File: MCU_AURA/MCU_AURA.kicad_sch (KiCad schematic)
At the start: 0 parts

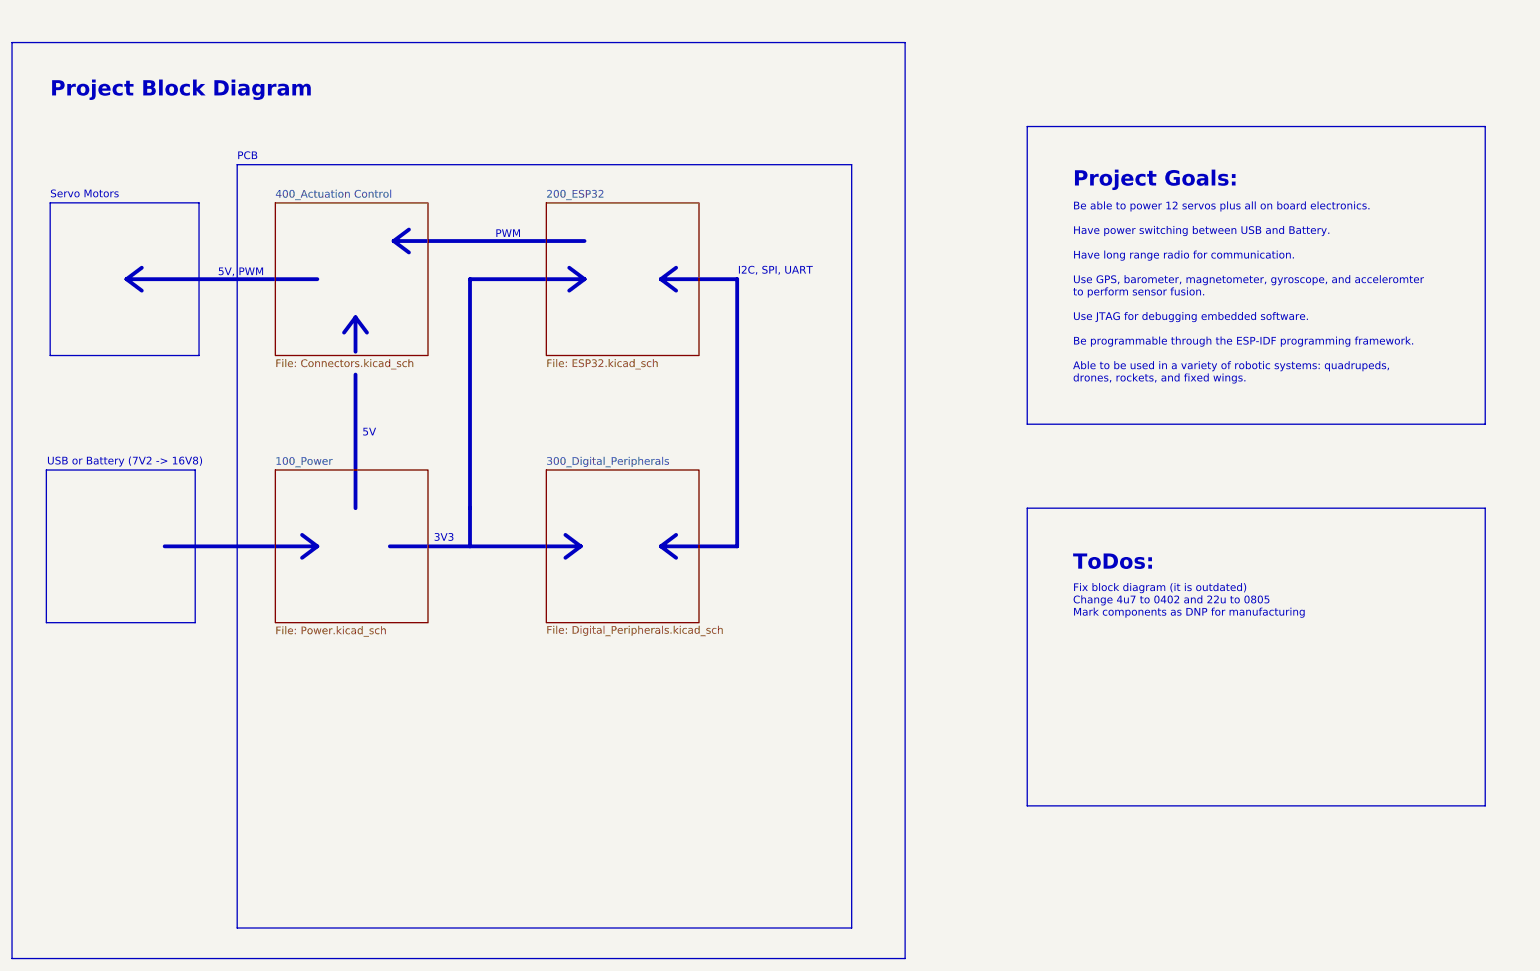
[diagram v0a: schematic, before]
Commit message: First fully routed version
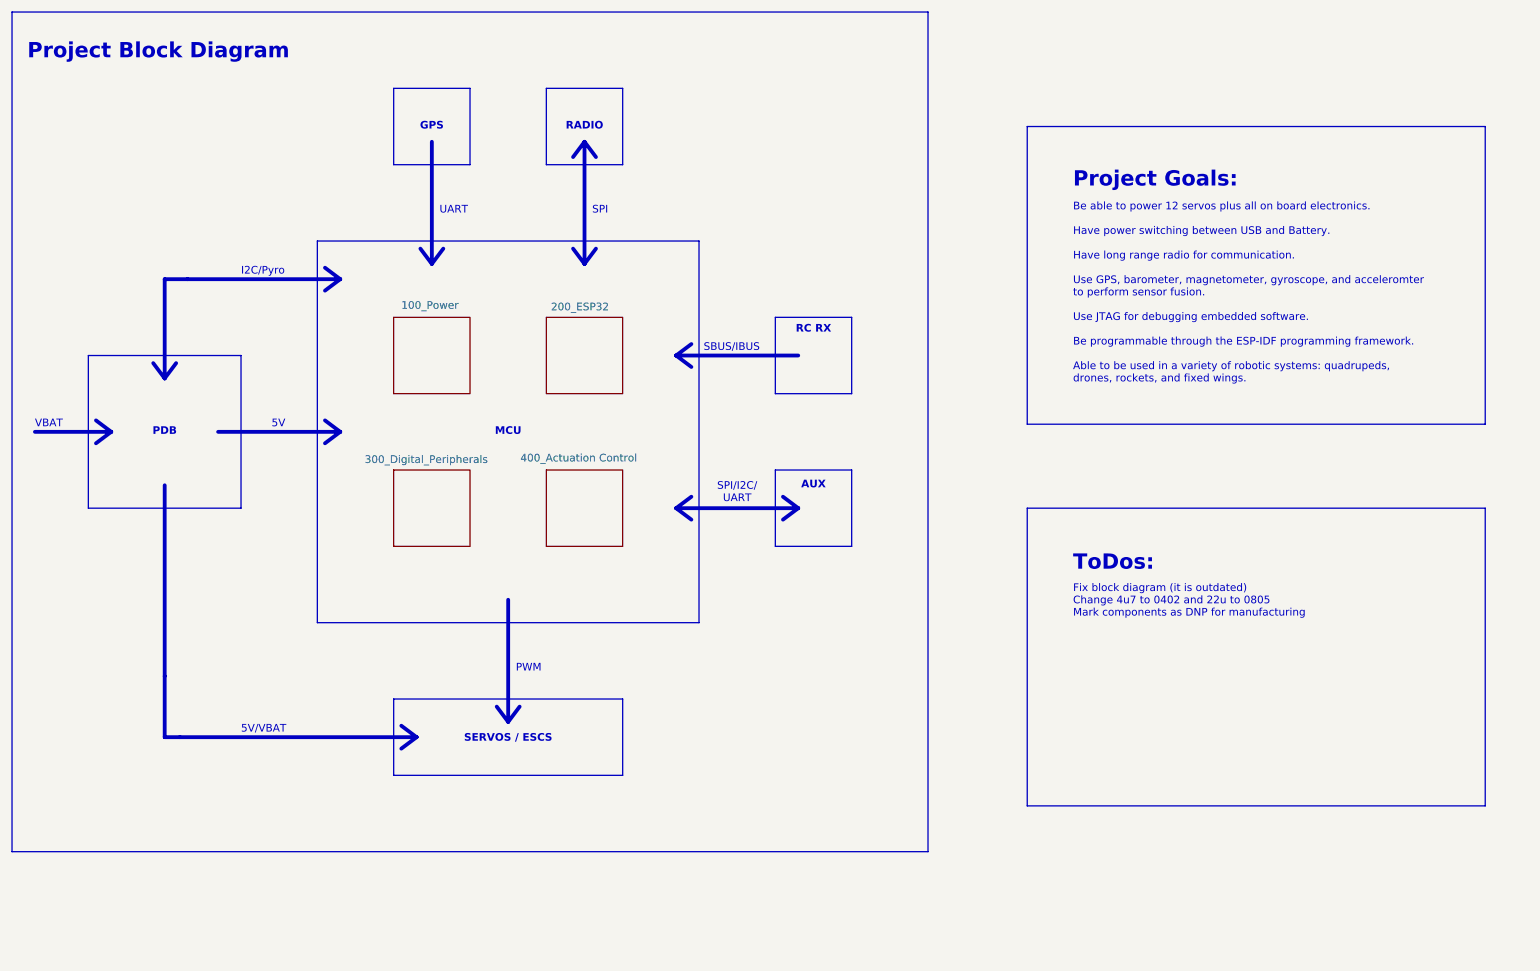
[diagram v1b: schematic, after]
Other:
- note added: "5V/VBAT"
- note added: "AUX"
- note added: "GPS"
- note added: "I2C/Pyro"
- note added: "MCU"
- note added: "PDB"
- note added: "RADIO"
- note added: "RC RX"
- note added: "SBUS/IBUS"
- note added: "SERVOS / ESCS"
- note added: "SPI"
- note added: "SPI/I2C/ UART"
- note added: "UART"
- note added: "VBAT"
- note removed: "3V3"
- note removed: "5V, PWM"
- note removed: "I2C, SPI, UART"
- note removed: "PCB"
- note removed: "Servo Motors"
- note removed: "USB or Battery (7V2 -> 16V8)"
